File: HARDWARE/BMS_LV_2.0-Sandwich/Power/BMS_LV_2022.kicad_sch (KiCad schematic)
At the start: 11 parts, among them J1 Conn_01x26, J2 AS214-97PN, J4 Battery+, J5 Battery-

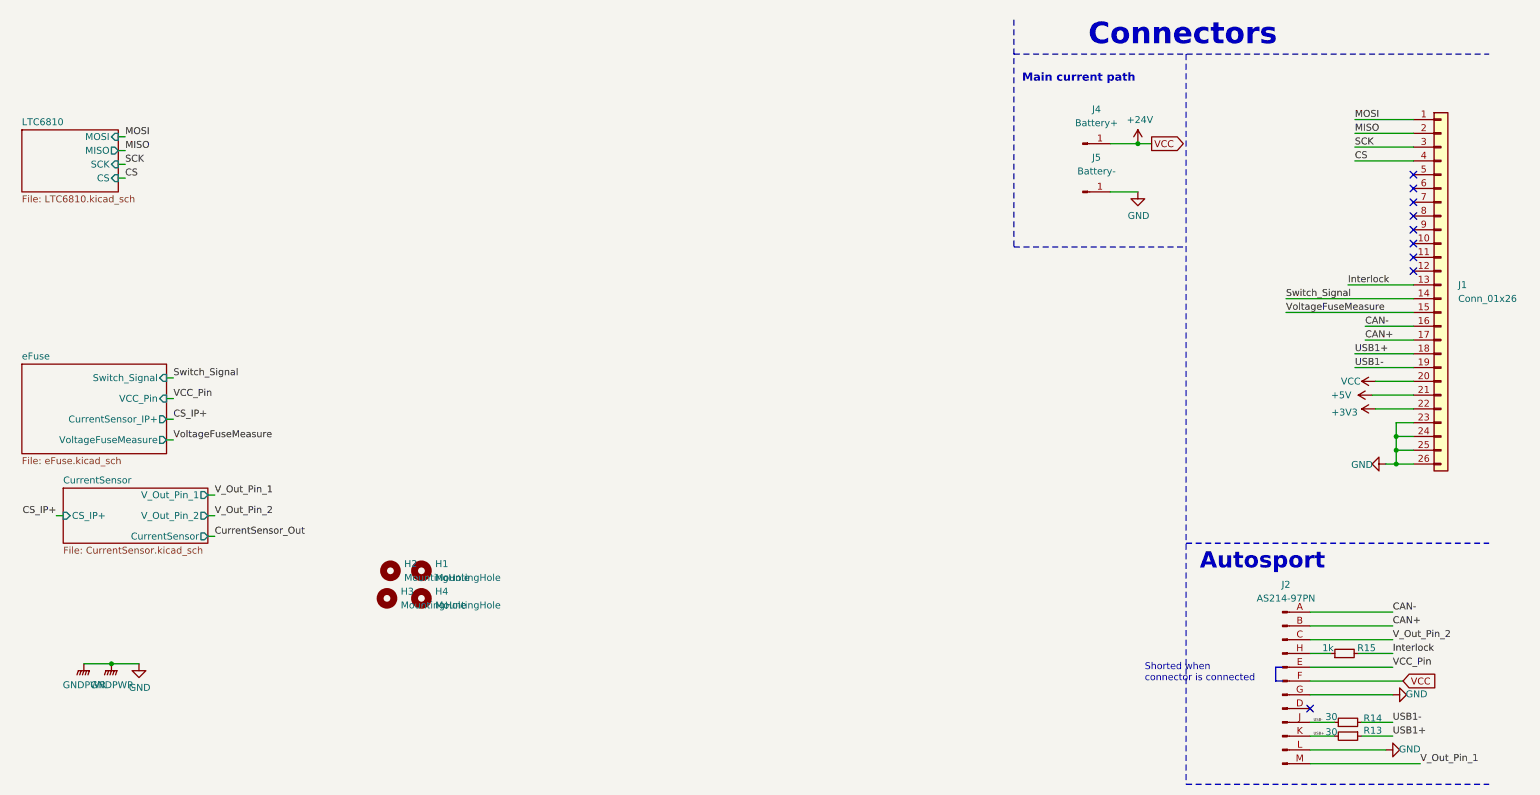
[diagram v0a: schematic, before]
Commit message: V1.0 ready for release
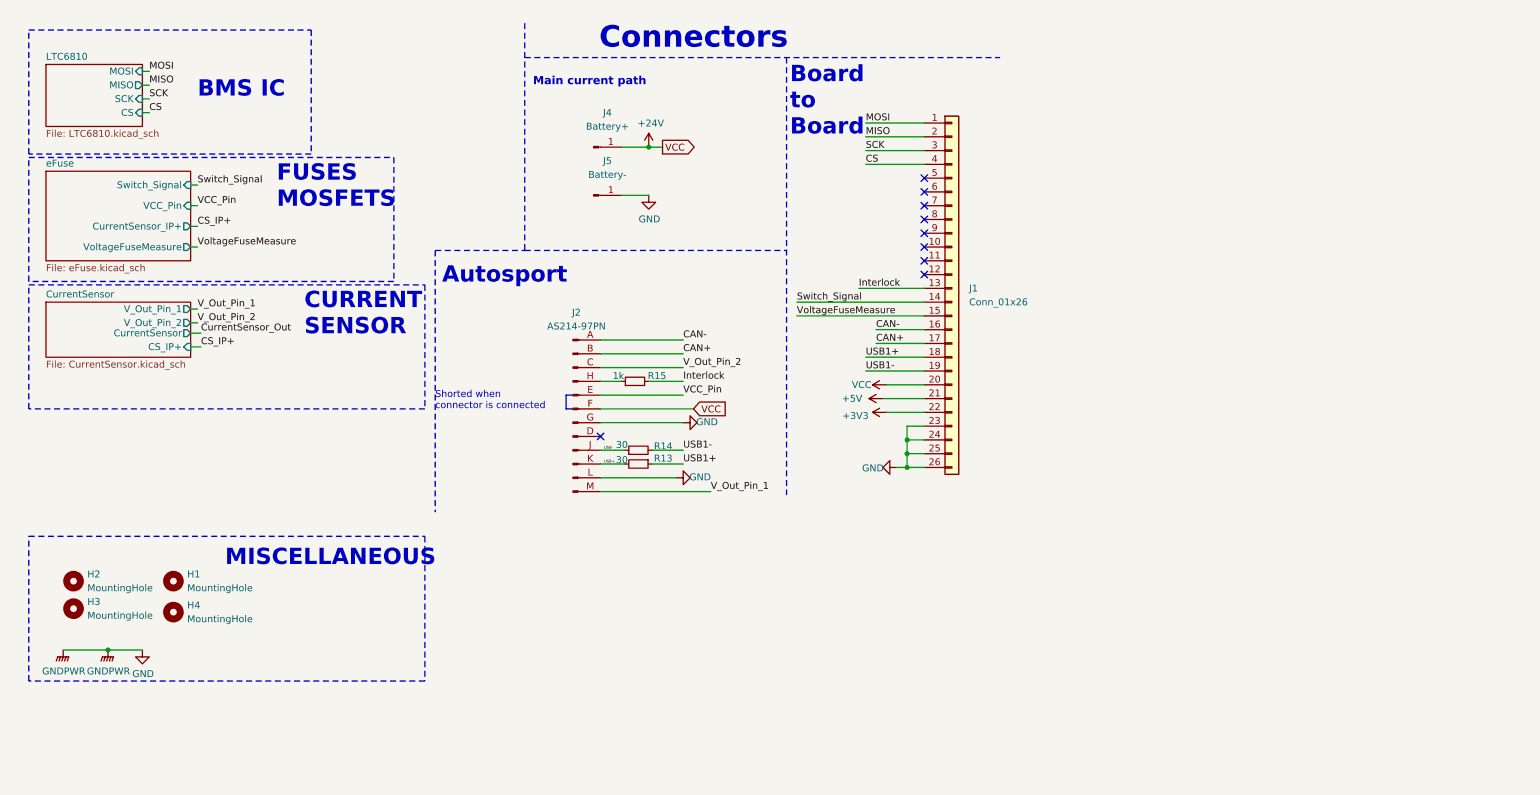
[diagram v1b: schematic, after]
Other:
- note added: "BMS IC"
- note added: "Board to Board"
- note added: "CURRENT SENSOR"
- note added: "FUSES MOSFETS"
- note added: "MISCELLANEOUS"
- moved on the sheet: H1, H2, H3, H4, J1, J2, J4, J5, R13, R14, R15
